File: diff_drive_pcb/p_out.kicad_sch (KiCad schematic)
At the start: 10 parts, among them J12 5v_out_1, J13 5v_out_2, J14 5v_out_3, J15 5v_out_4, J16 3v3_out_1, J17 3v3_out_2, J18 3v3_out_3, J19 3v3_out_4

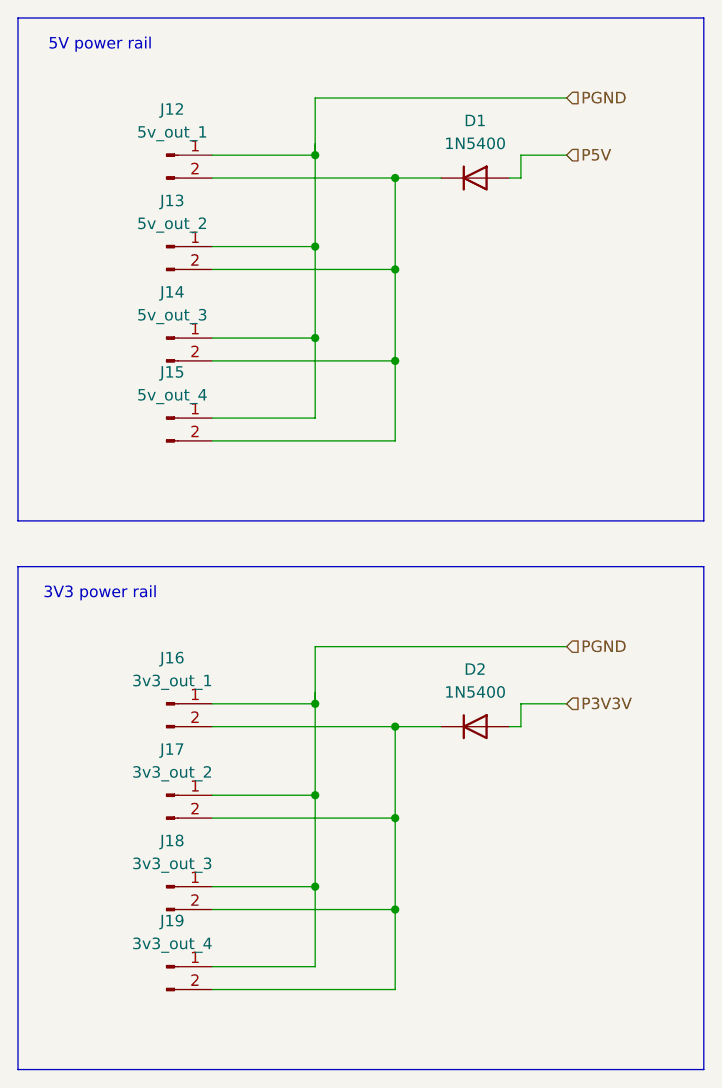
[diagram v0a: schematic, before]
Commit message: Updated Schematic
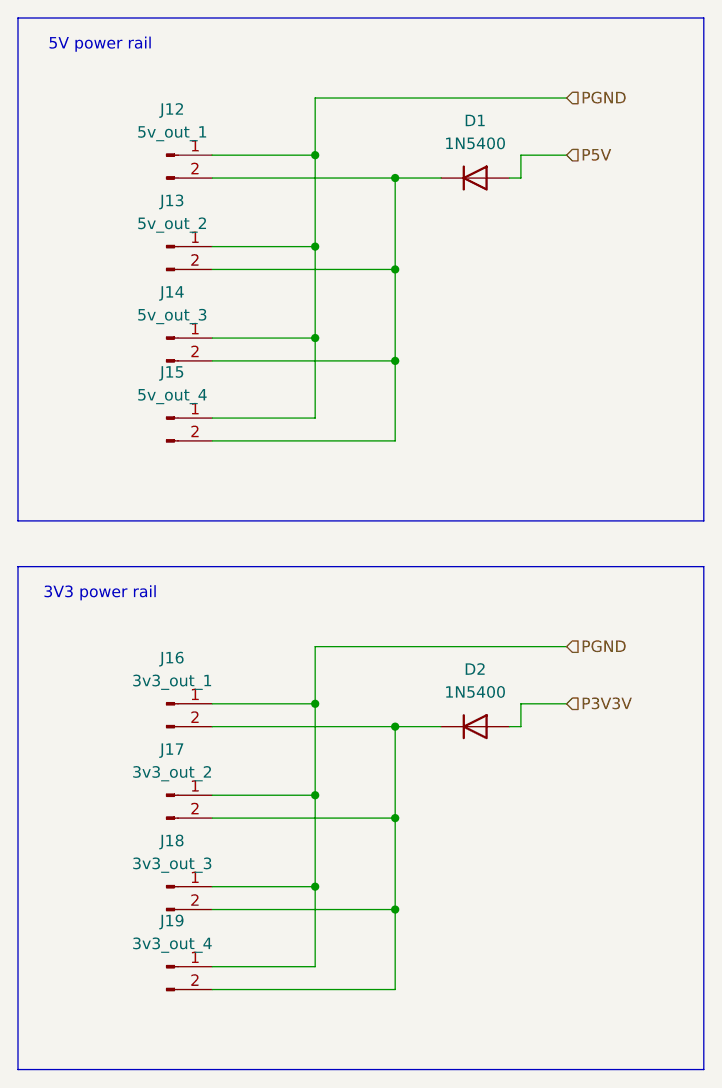
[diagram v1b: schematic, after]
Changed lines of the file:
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@@
-	(wire
-		(pts
-			(xy 82.55 101.6) (xy 82.55 100.33)
-		)
-		(stroke
-			(width 0)
-			(type default)
-		)
-	)
 	(wire
 		(pts
@@
 		)
 	)
-	(wire
-		(pts
-			(xy 82.55 40.64) (xy 82.55 39.37)
-		)
-		(stroke
-			(width 0)
-			(type default)
-		)
-	)
